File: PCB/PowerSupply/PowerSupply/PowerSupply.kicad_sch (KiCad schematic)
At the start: 0 parts

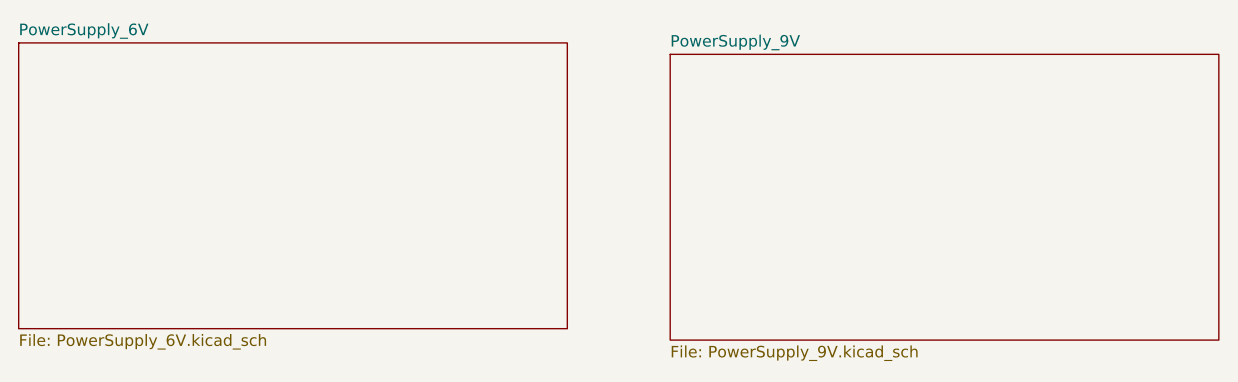
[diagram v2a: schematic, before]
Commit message: Finished v0.1
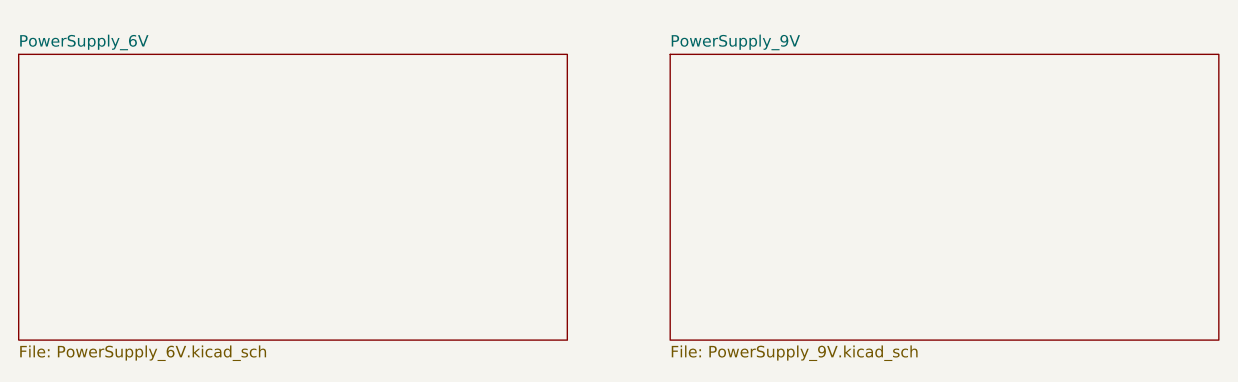
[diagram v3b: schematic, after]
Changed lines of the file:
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@@
     )
   )
-  (sheet (at 25.4 16.51) (size 60.96 31.75) (fields_autoplaced)
+  (sheet (at 25.4 17.78) (size 60.96 31.75) (fields_autoplaced)
     (stroke (width 0.1524) (type solid) (color 0 0 0 0))
     (fill (color 0 0 0 0.0000))
-    (property "Sheet name" "PowerSupply_6V" (id 0) (at 25.4 15.7984 0)
+    (property "Sheet name" "PowerSupply_6V" (id 0) (at 25.4 17.0684 0)
       (effects (font (size 1.27 1.27)) (justify left bottom))
     )
-    (property "Sheet file" "PowerSupply_6V.kicad_sch" (id 1) (at 25.4 48.8446 0)
+    (property "Sheet file" "PowerSupply_6V.kicad_sch" (id 1) (at 25.4 50.1146 0)
       (effects (font (size 1.27 1.27)) (justify left top))
     )
@@
   )
   (symbol_instances
+    (path "/d52e6e97-797a-47f3-9e84-2594d0785aa0/66d410c0-7cfb-449e-9a14-33526c090e49"
+      (reference "#FLG0101") (unit 1) (value "PWR_FLAG") (footprint "")
+    )
     (path "/d52e6e97-797a-47f3-9e84-2594d0785aa0/a6cca68e-2819-49c2-af51-6d2a54e1615b"
       (reference "#PWR0101") (unit 1) (value "GND") (footprint "")
@@
       (reference "#PWR0104") (unit 1) (value "GND") (footprint "")
     )
+    (path "/d52e6e97-797a-47f3-9e84-2594d0785aa0/eb233b0f-a872-4930-aedf-8c6d215fd56e"
+      (reference "#PWR0105") (unit 1) (value "GND") (footprint "")
+    )
     (path "/d52e6e97-797a-47f3-9e84-2594d0785aa0/408f320a-98fc-43da-b743-5ca46a73fedb"
